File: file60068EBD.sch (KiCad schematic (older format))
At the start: 0 parts

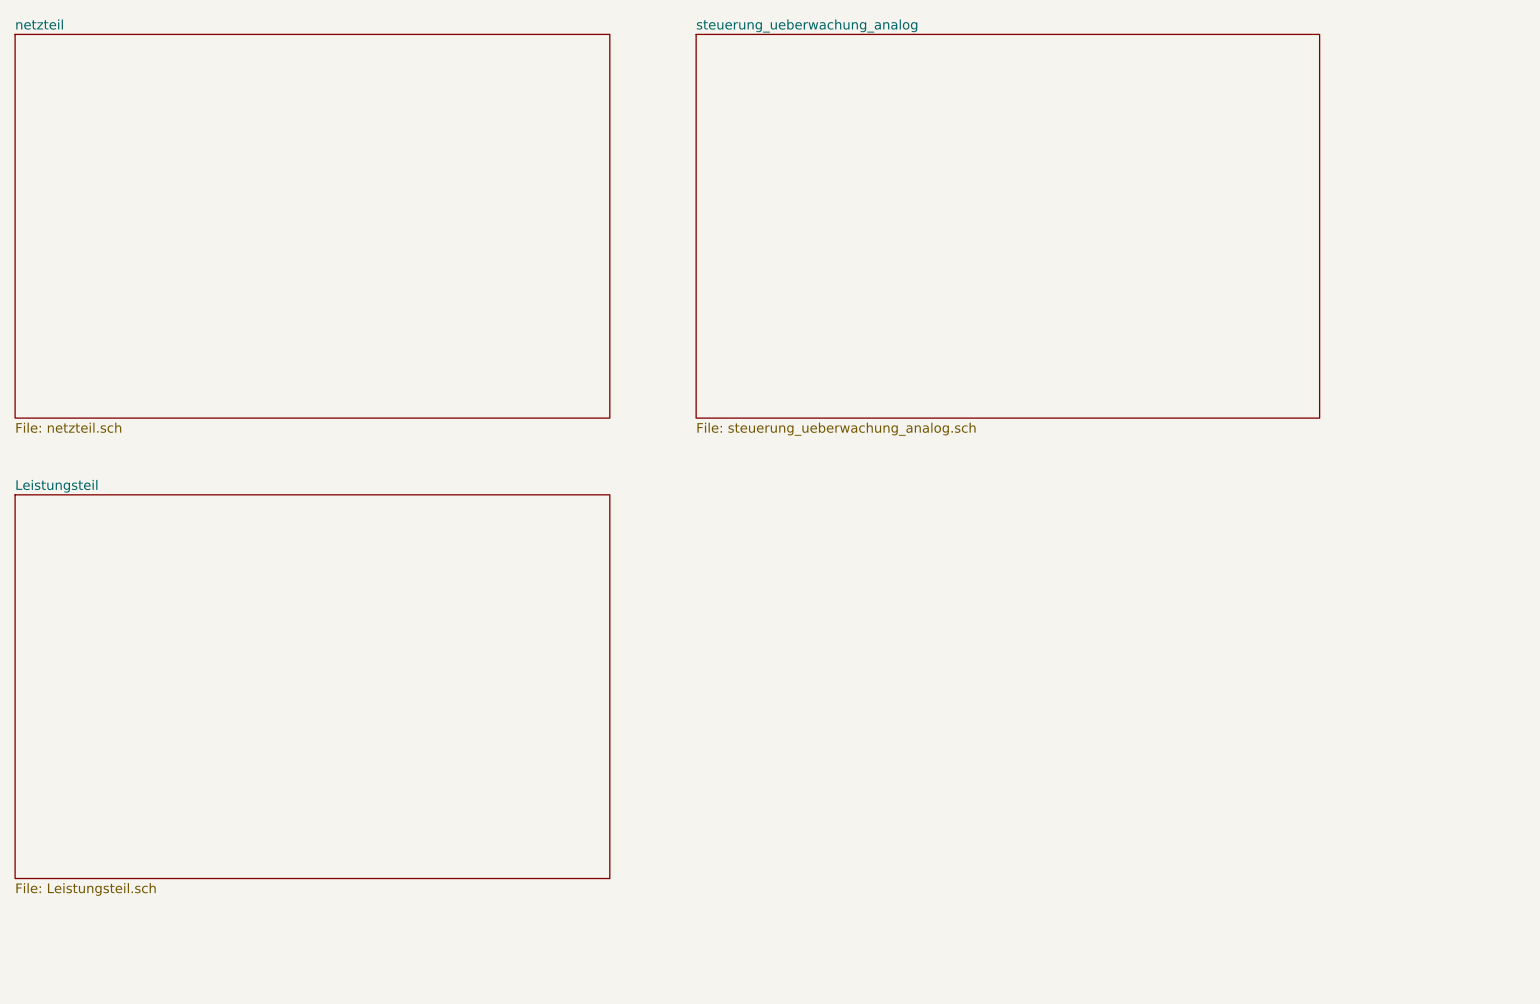
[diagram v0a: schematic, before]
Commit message: revision of Netzteil
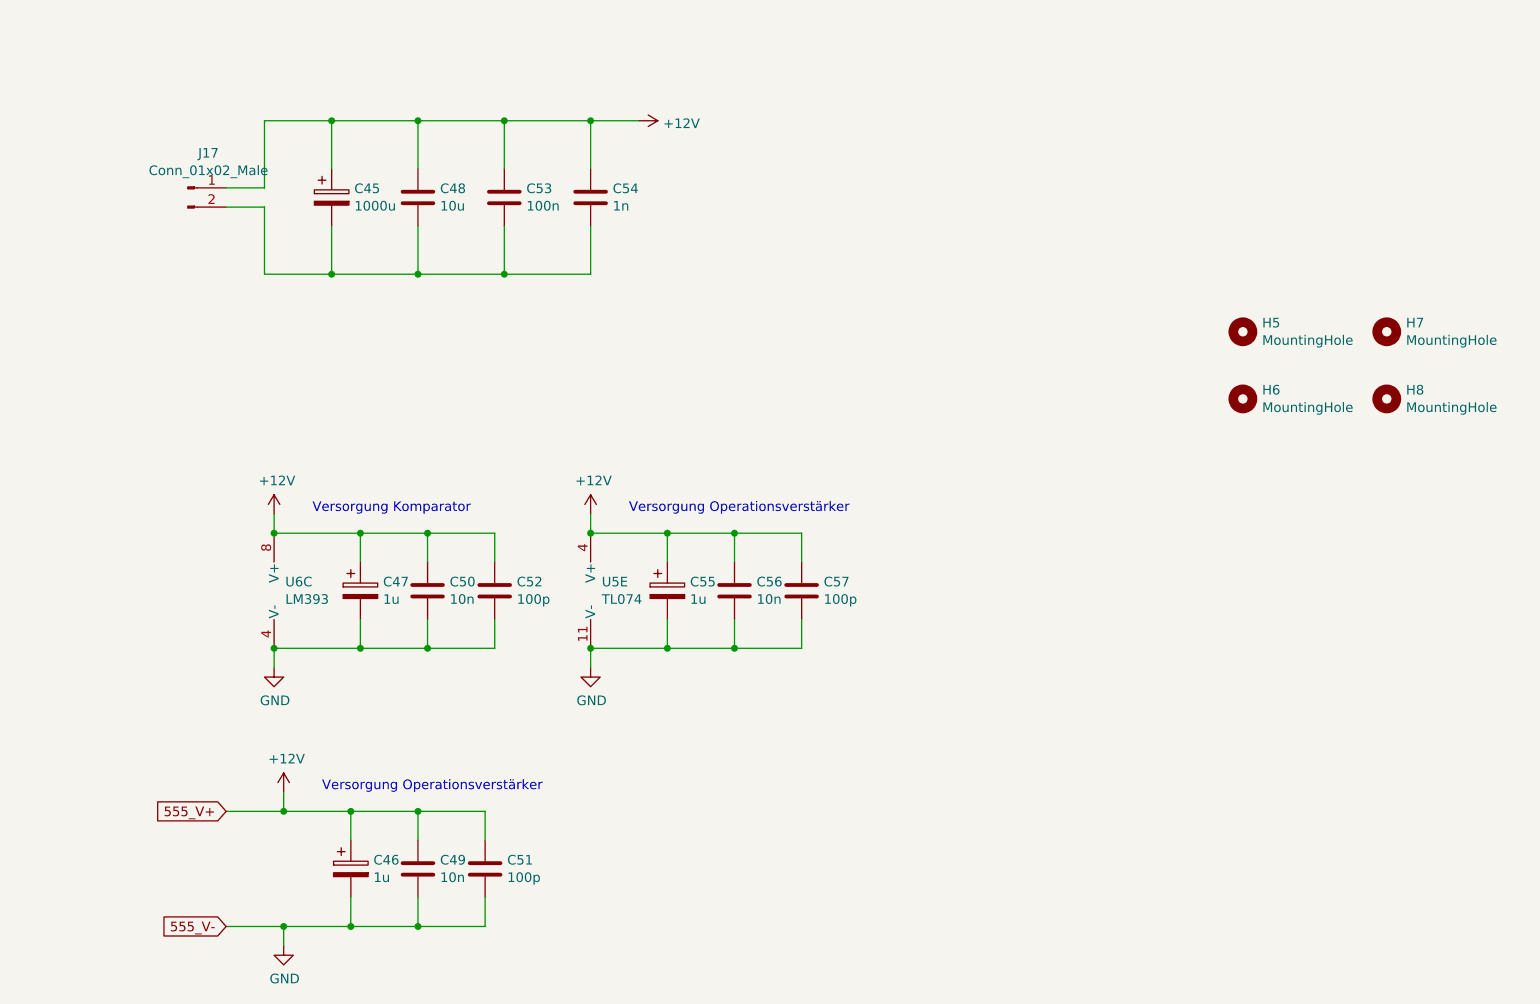
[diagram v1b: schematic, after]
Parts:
- added C45: 1000u, Capacitor_THT:CP_Radial_D5.0mm_P2.50mm, symbol Device:CP
- added C46, C47, C55: 1u, Capacitor_THT:CP_Radial_D5.0mm_P2.50mm, symbol Device:CP
- added C48: 10u, Capacitor_THT:C_Disc_D10.5mm_W5.0mm_P10.00mm, symbol Device:C
- added C49, C50, C56: 10n, Capacitor_THT:C_Disc_D10.0mm_W2.5mm_P5.00mm, symbol Device:C
- added C51, C52, C57: 100p, Capacitor_THT:C_Disc_D10.0mm_W2.5mm_P5.00mm, symbol Device:C
- added C53: 100n, Capacitor_THT:C_Disc_D10.5mm_W5.0mm_P10.00mm, symbol Device:C
- added C54: 1n, Capacitor_THT:C_Disc_D10.5mm_W5.0mm_P10.00mm, symbol Device:C
- added H5, H6, H7, H8: MountingHole, MountingHole:MountingHole_2.7mm, symbol Mechanical:MountingHole
- added J17: Conn_01x02_Male, symbol Connector:Conn_01x02_Male
- added U5: TL074, symbol Amplifier_Operational:TL074
- added U6: LM393, digikey-footprints:DIP-8_W7.62mm, symbol Comparator:LM393
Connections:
- new net: C45.2, C48.2, C53.2, C54.2, J17.2 (Pin_2)
- new net +12V: C45.1, C46.1, C47.1, C48.1, C49.1, C50.1, C51.1, C52.1, C53.1, C54.1, C55.1, C56.1, C57.1, J17.1 (Pin_1), U5.4 (V+), U6.8 (V+)
- new net GND: C46.2, C47.2, C49.2, C50.2, C51.2, C52.2, C55.2, C56.2, C57.2, U5.11 (V-), U6.4 (V-)
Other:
- note added: "Versorgung Komparator"
- note added: "Versorgung Operationsverstärker"
